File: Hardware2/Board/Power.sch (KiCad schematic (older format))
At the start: 41 parts, among them J4 J, J5 J, J6 J, P20 TP, P21 TP, P22 TP, P23 TP, P24 2060-452, P25 2060-452, P26 TP, P27 TP, P28 2060-452, P29 2059-302, P30 LED_Strip, P31 LED_Strip, U5 TPS82130, U6 LP2985IM5-3.3, U7 TPS82130, U8 SP485CN, U9 TPS82130

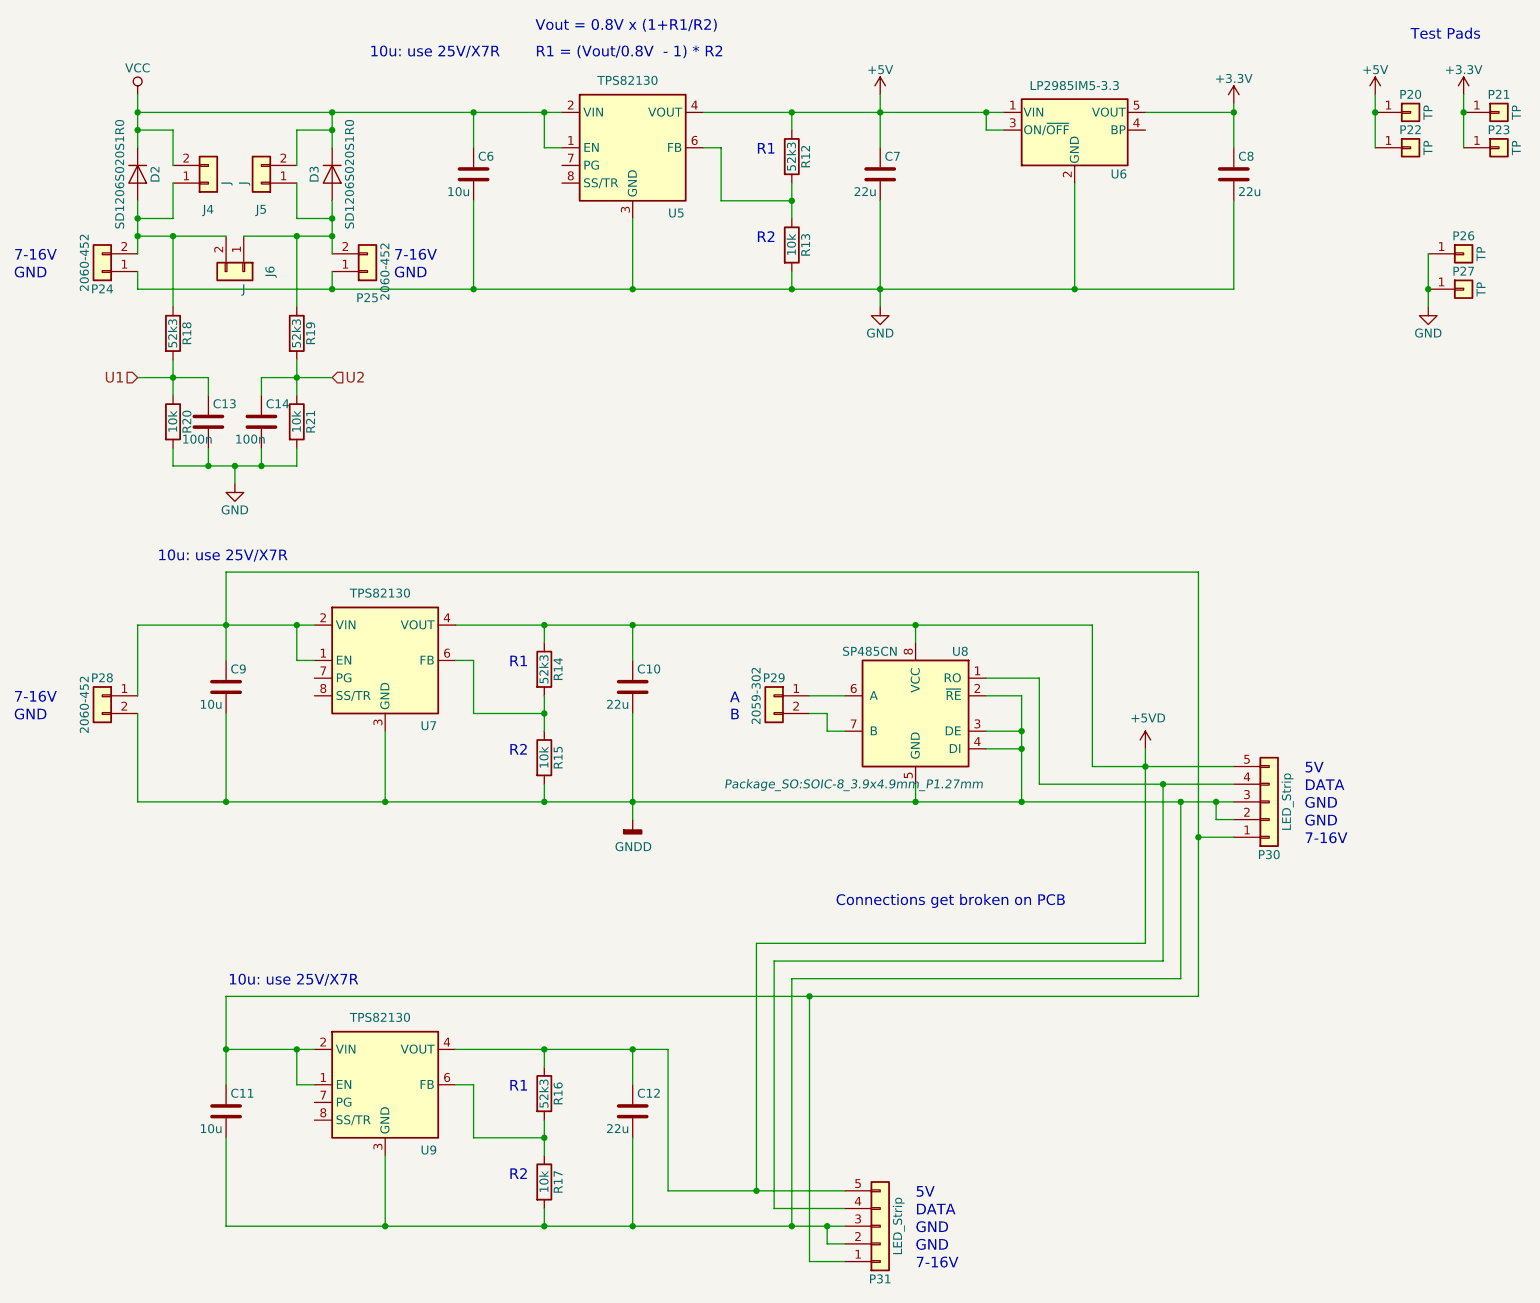
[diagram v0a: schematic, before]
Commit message: Add CAN bus
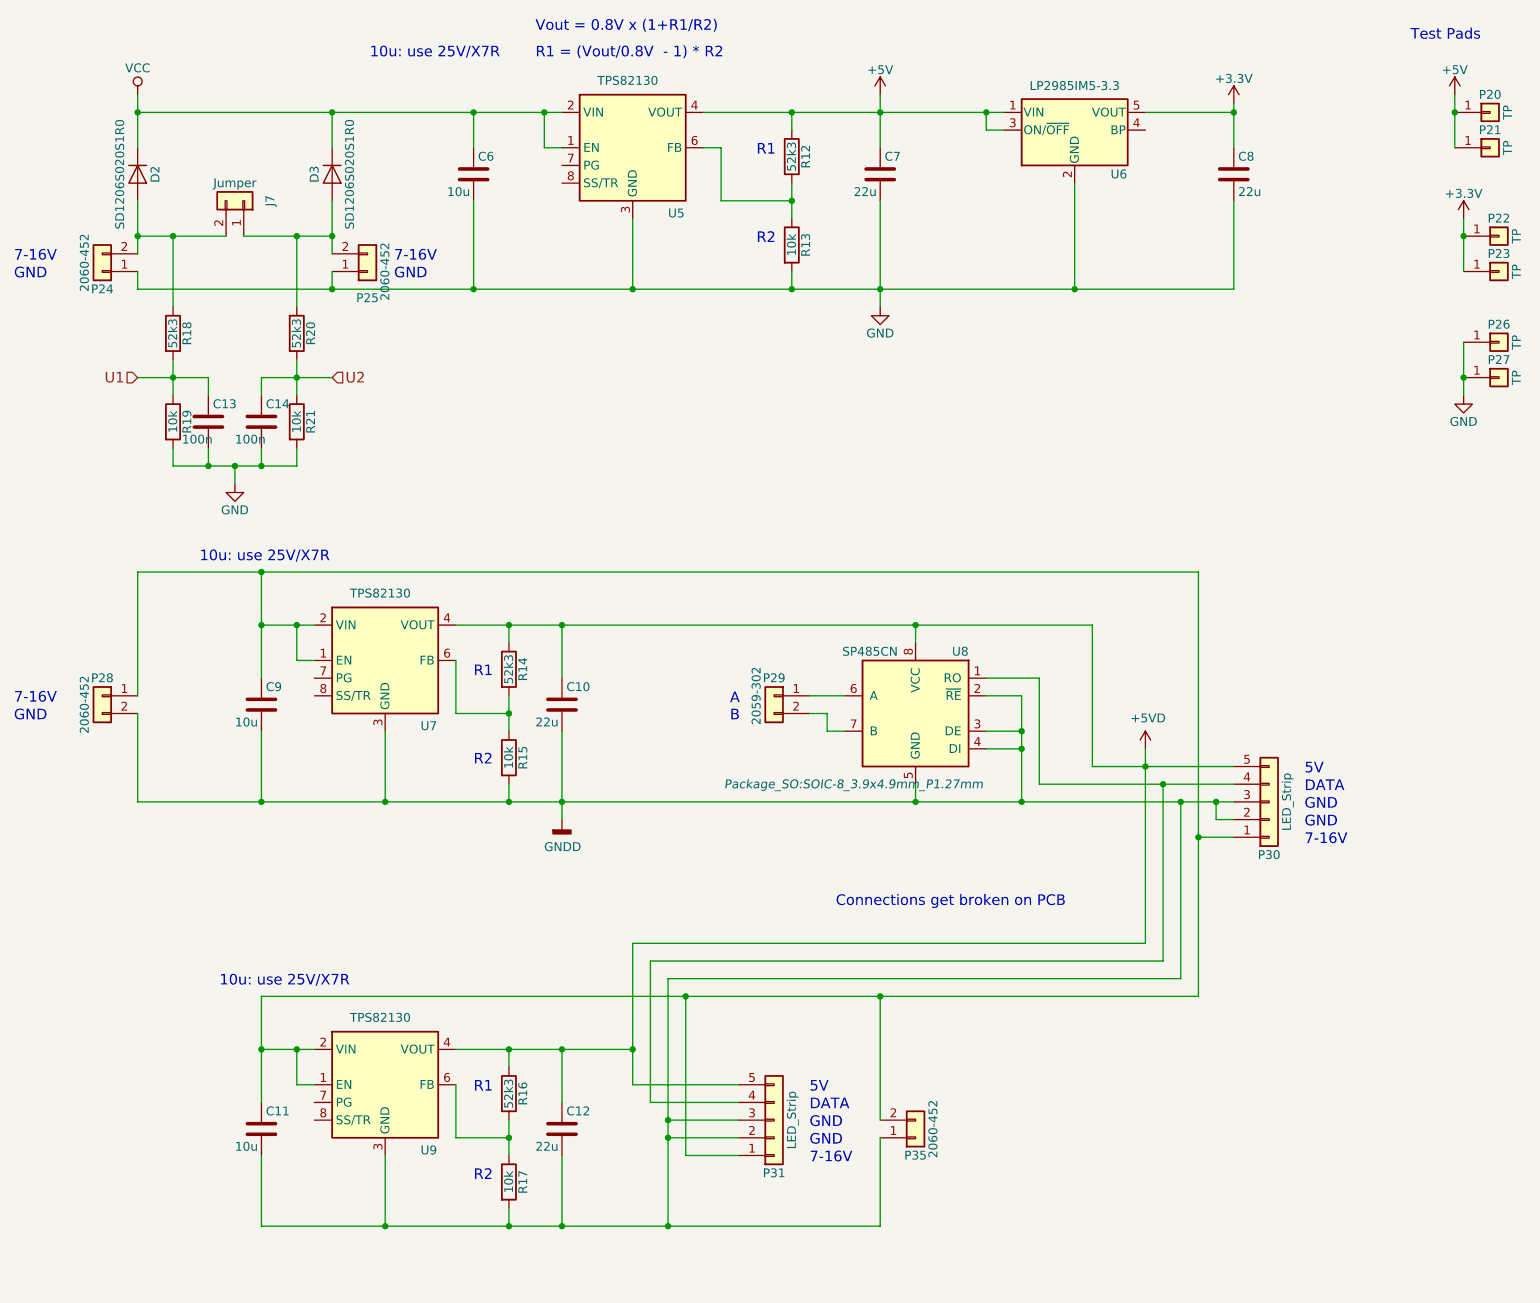
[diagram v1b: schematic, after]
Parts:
- removed J4, J5: J, LedControl:Jumper, symbol Connector_Generic:Conn_01x02
- added P35: 2060-452, LedControl:WAGO_2060-452, symbol Connector_Generic:Conn_01x02
- J7: renamed from J6; value J -> Jumper
- renumbered P22 to P21, P21 to P22, R20 to R19, R19 to R20
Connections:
- net GNDD: now also P35.1 (Pin_1)
- net at C11.1, C9.1, P28.1 (Pin_1)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: now also P35.2 (Pin_2)
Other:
- moved on the sheet: C10, C11, C12, C9, J7, P20, P21, P22, P23, P26, P27, P31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
